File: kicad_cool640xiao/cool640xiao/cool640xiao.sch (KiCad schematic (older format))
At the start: 49 parts, among them J1 MJ-4PP-9, J2 MJ-4PP-9, J3 MJ-4PP-9, J4 MJ-4PP-9, SW1 SW_PUSH, SW10 SW_PUSH, SW11 SW_PUSH, SW12 SW_PUSH, SW13 SW_PUSH, SW14 SW_PUSH, SW15 SW_PUSH, SW16 SW_PUSH, SW17 SW_PUSH, SW18 SW_PUSH, SW19 SW_PUSH, SW2 SW_PUSH, SW20 SW_PUSH, SW21 Rotary_Encoder_Switch, SW22 Rotary_Encoder_Switch, SW3 SW_PUSH, SW4 SW_PUSH, SW5 SW_PUSH, SW6 SW_PUSH, SW7 SW_PUSH, SW8 SW_PUSH, SW9 SW_PUSH, U1 SeeeduinoXIAO

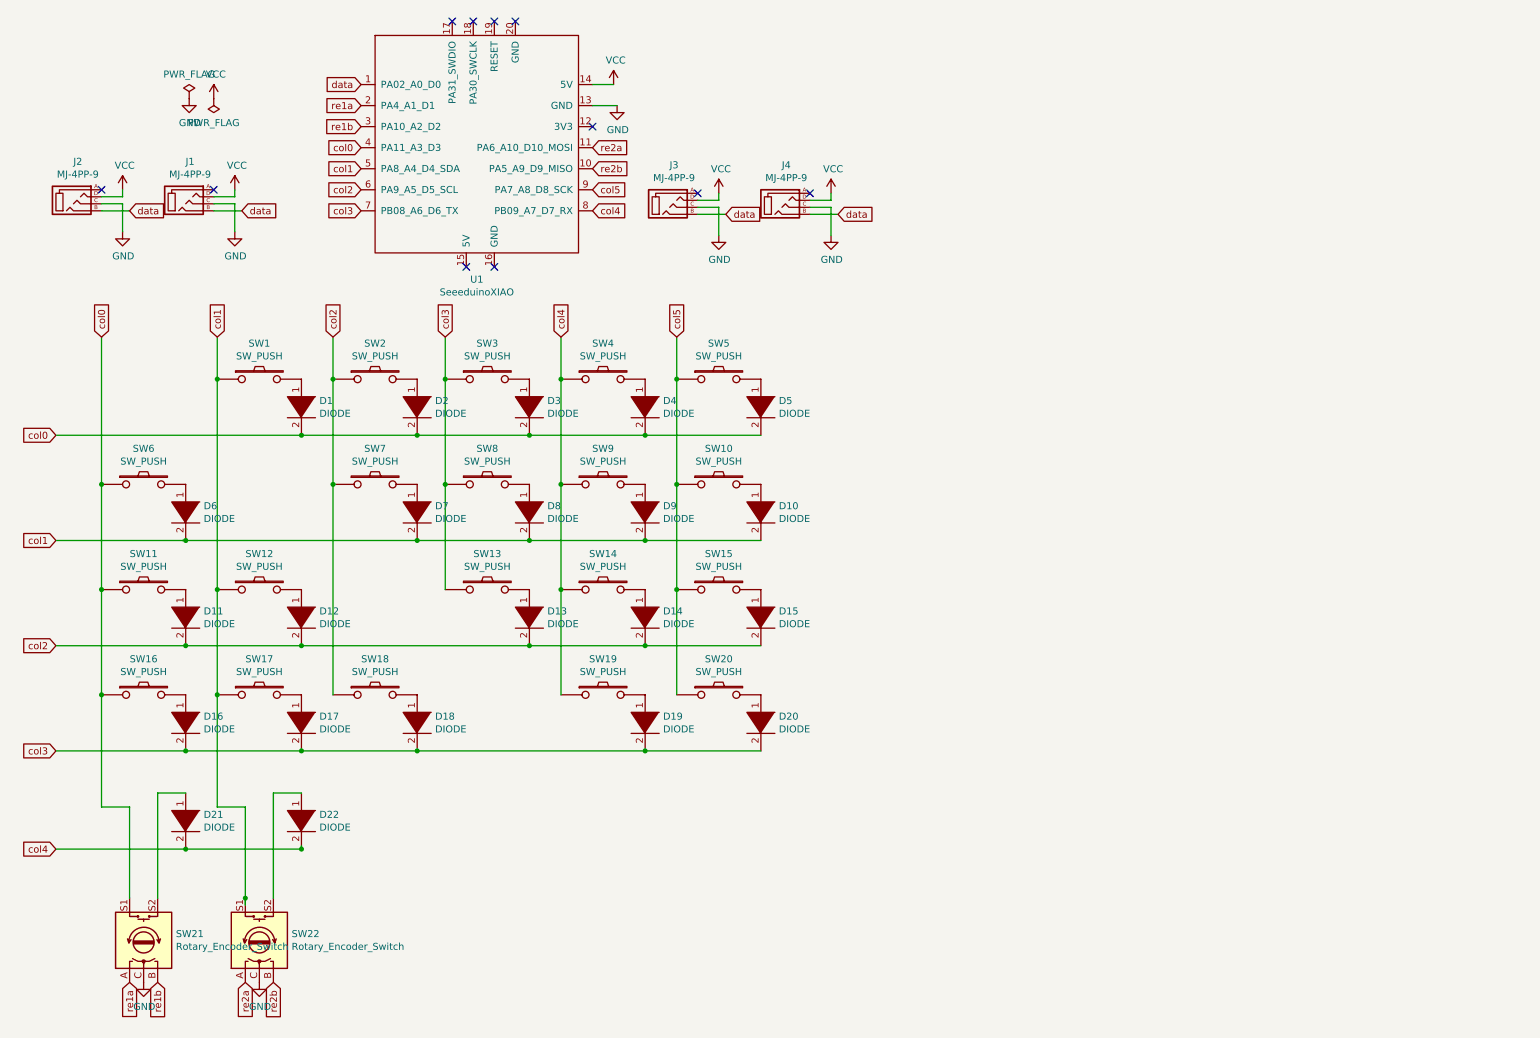
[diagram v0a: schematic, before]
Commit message: fix
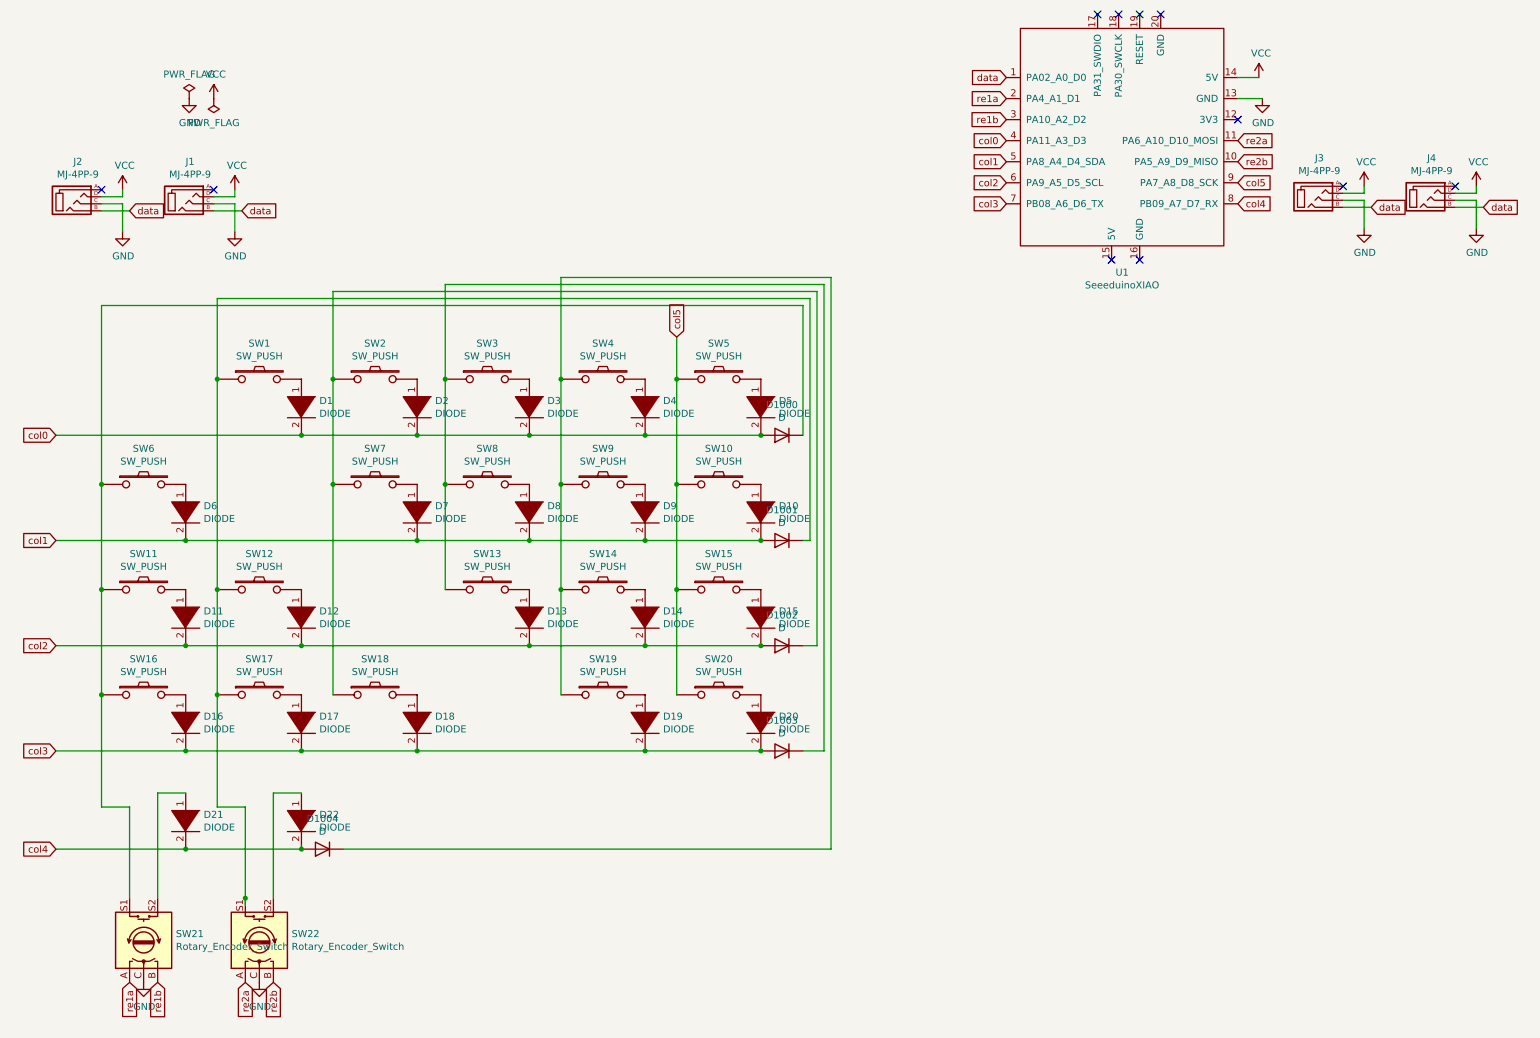
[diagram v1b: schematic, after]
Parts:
- added D1000, D1001, D1002, D1003, D1004: D, kbd:D3_TH_SMD, symbol Device:D
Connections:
- wire segments 77 -> 91
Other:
- moved on the sheet: J3, J4, U1
